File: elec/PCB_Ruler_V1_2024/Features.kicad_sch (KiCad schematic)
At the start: 4 parts

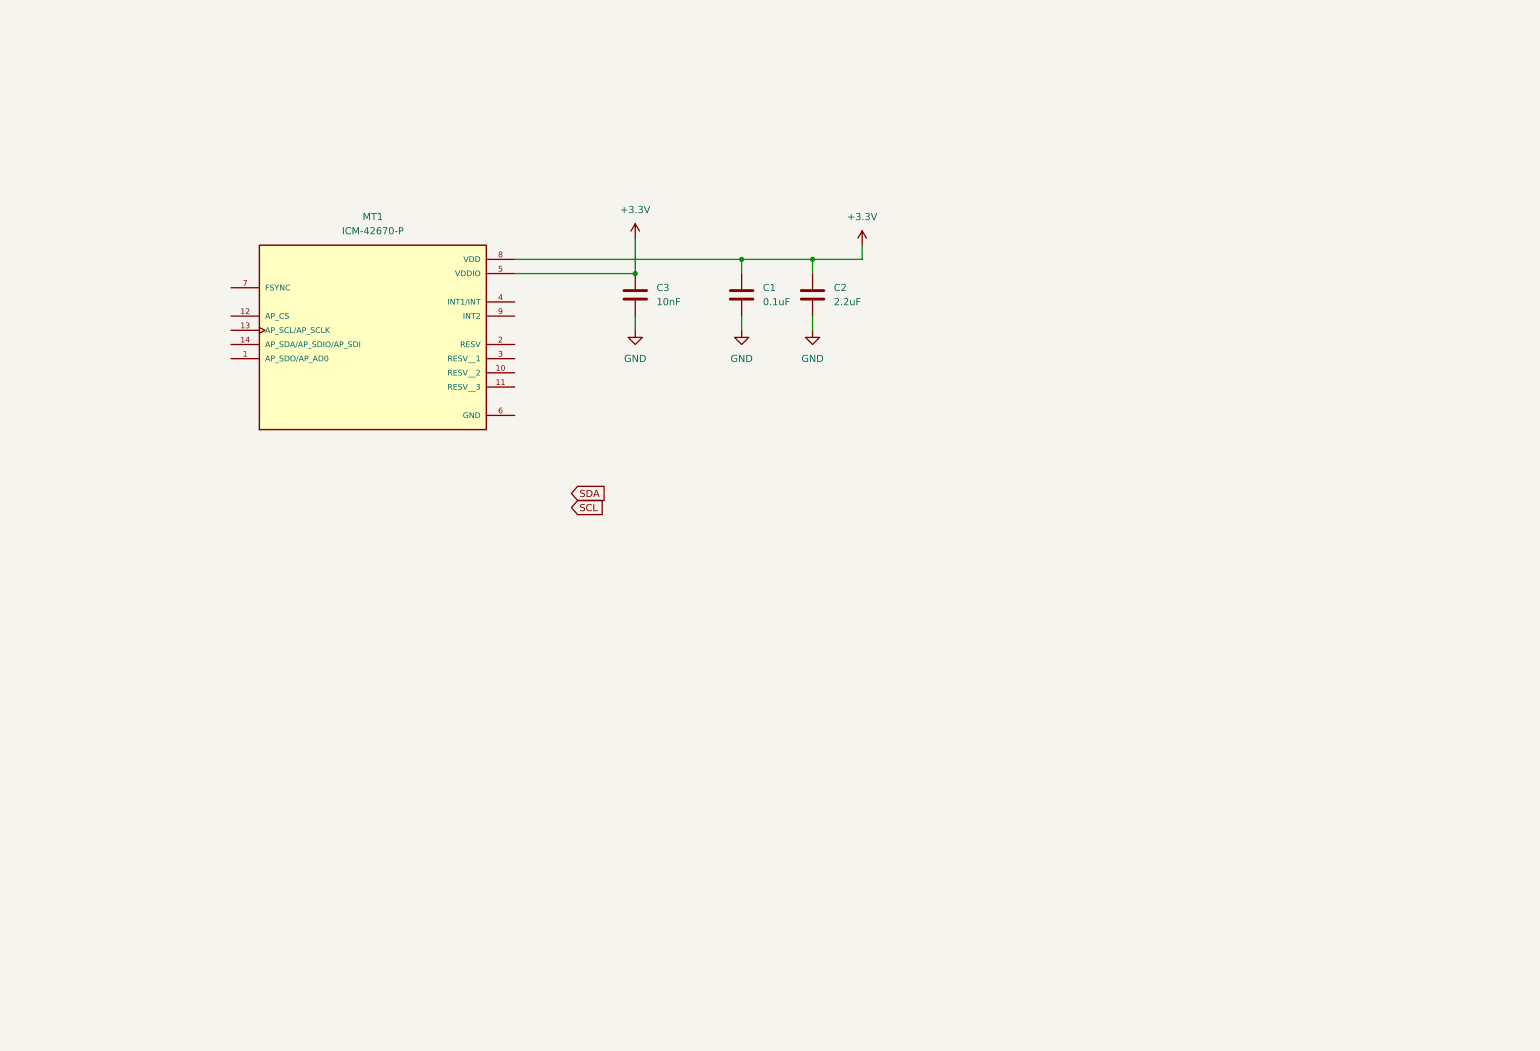
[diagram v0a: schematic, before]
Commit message: Laser
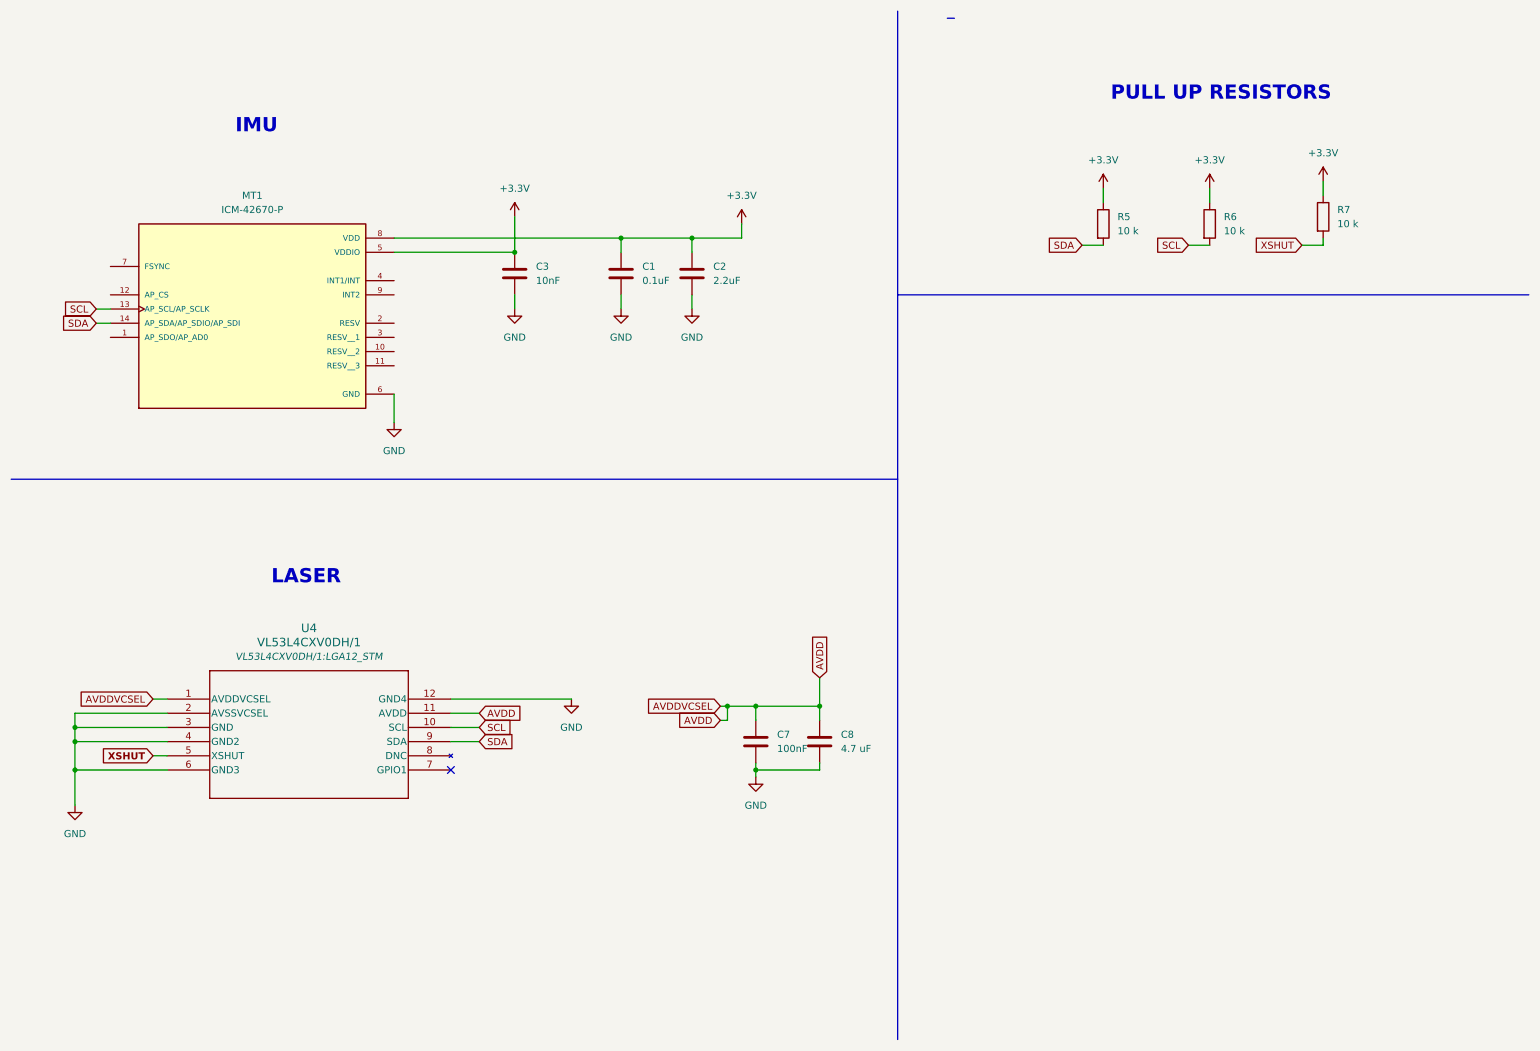
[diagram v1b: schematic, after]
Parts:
- added C7: 100nF, symbol Device:C
- added C8: 4.7 uF, symbol Device:C
- added R5, R6, R7: 10 k, symbol Device:R
- added U4: VL53L4CXV0DH/1, VL53L4CXV0DH/1:LGA12_STM, symbol VL53L4CXV0DH/1:VL53L4CXV0DH_1
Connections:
- net +3.3V: now also R5.1, R6.1, R7.1
- net GND: now also MT1.6 (GND), C7.2, C8.2, U4.12 (GND4), U4.2 (AVSSVCSEL), U4.3 (GND), U4.4 (GND2), U4.6 (GND3)
- net SCL: now also MT1.13 (AP_SCL/AP_SCLK), R6.2, U4.10 (SCL)
- net SDA: now also MT1.14 (AP_SDA/AP_SDIO/AP_SDI), R5.2, U4.9 (SDA)
- new net AVDD: C7.1, C8.1, U4.1 (AVDDVCSEL), U4.11 (AVDD)
- new net XSHUT: R7.2, U4.5 (XSHUT)
- no-connect marks 0 -> 1
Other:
- note added: "IMU"
- note added: "LASER"
- note added: "PULL UP RESISTORS"
- moved on the sheet: C1, C2, C3, MT1

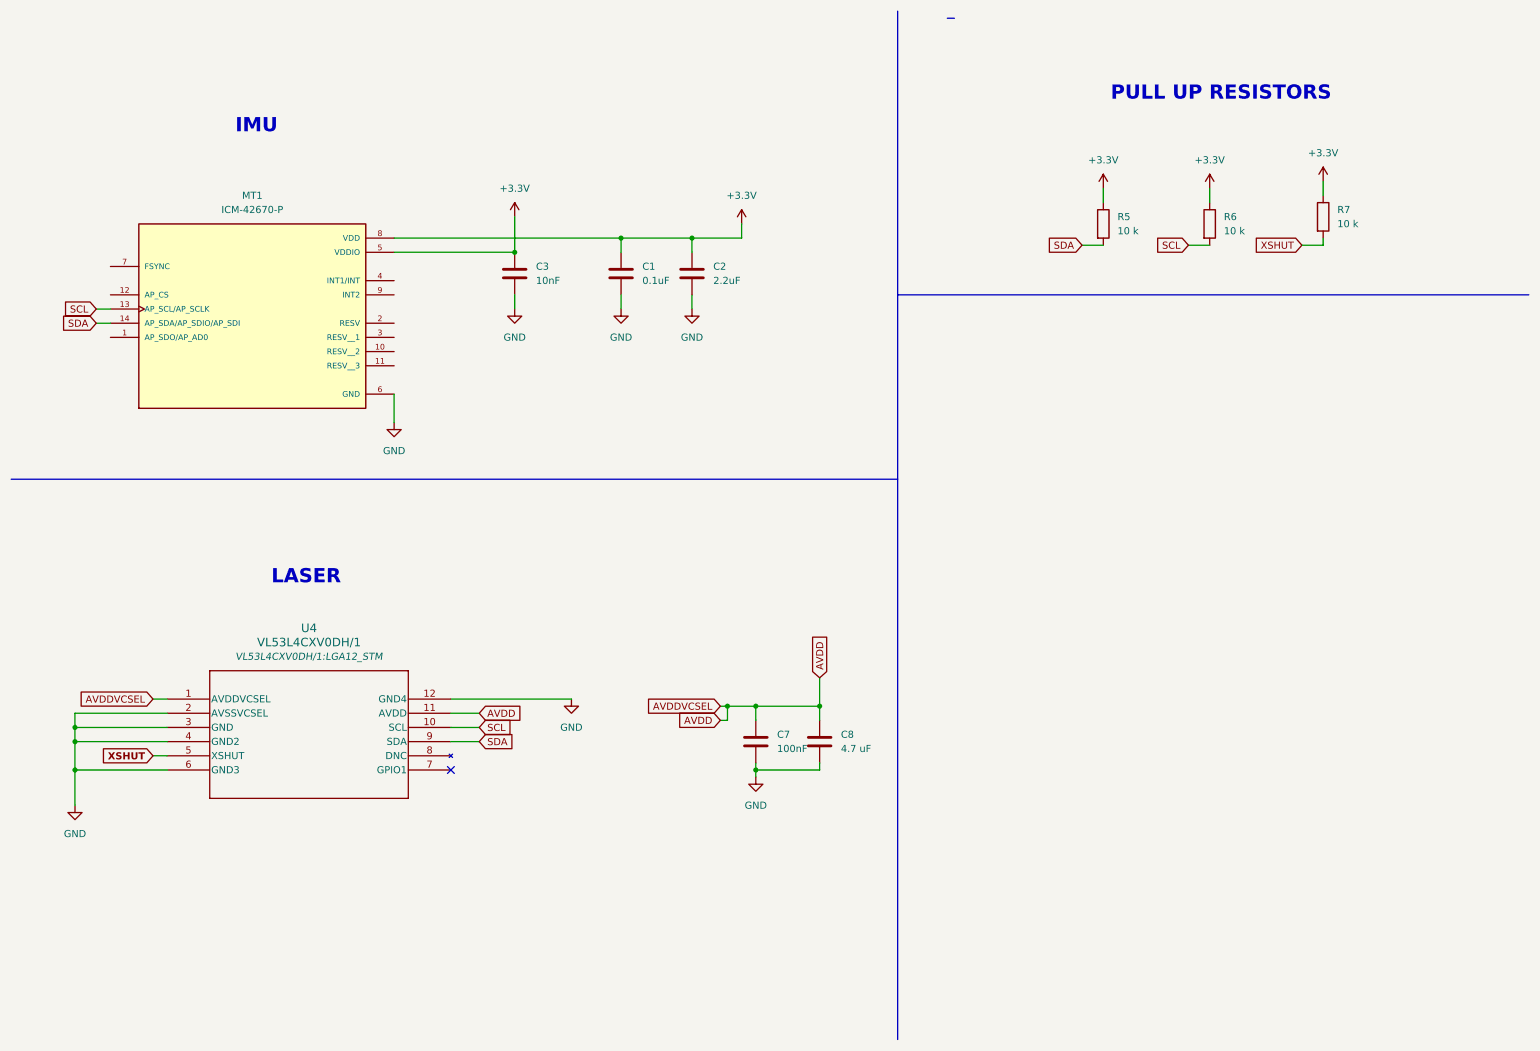
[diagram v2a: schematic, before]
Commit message: Almost finished schematic...
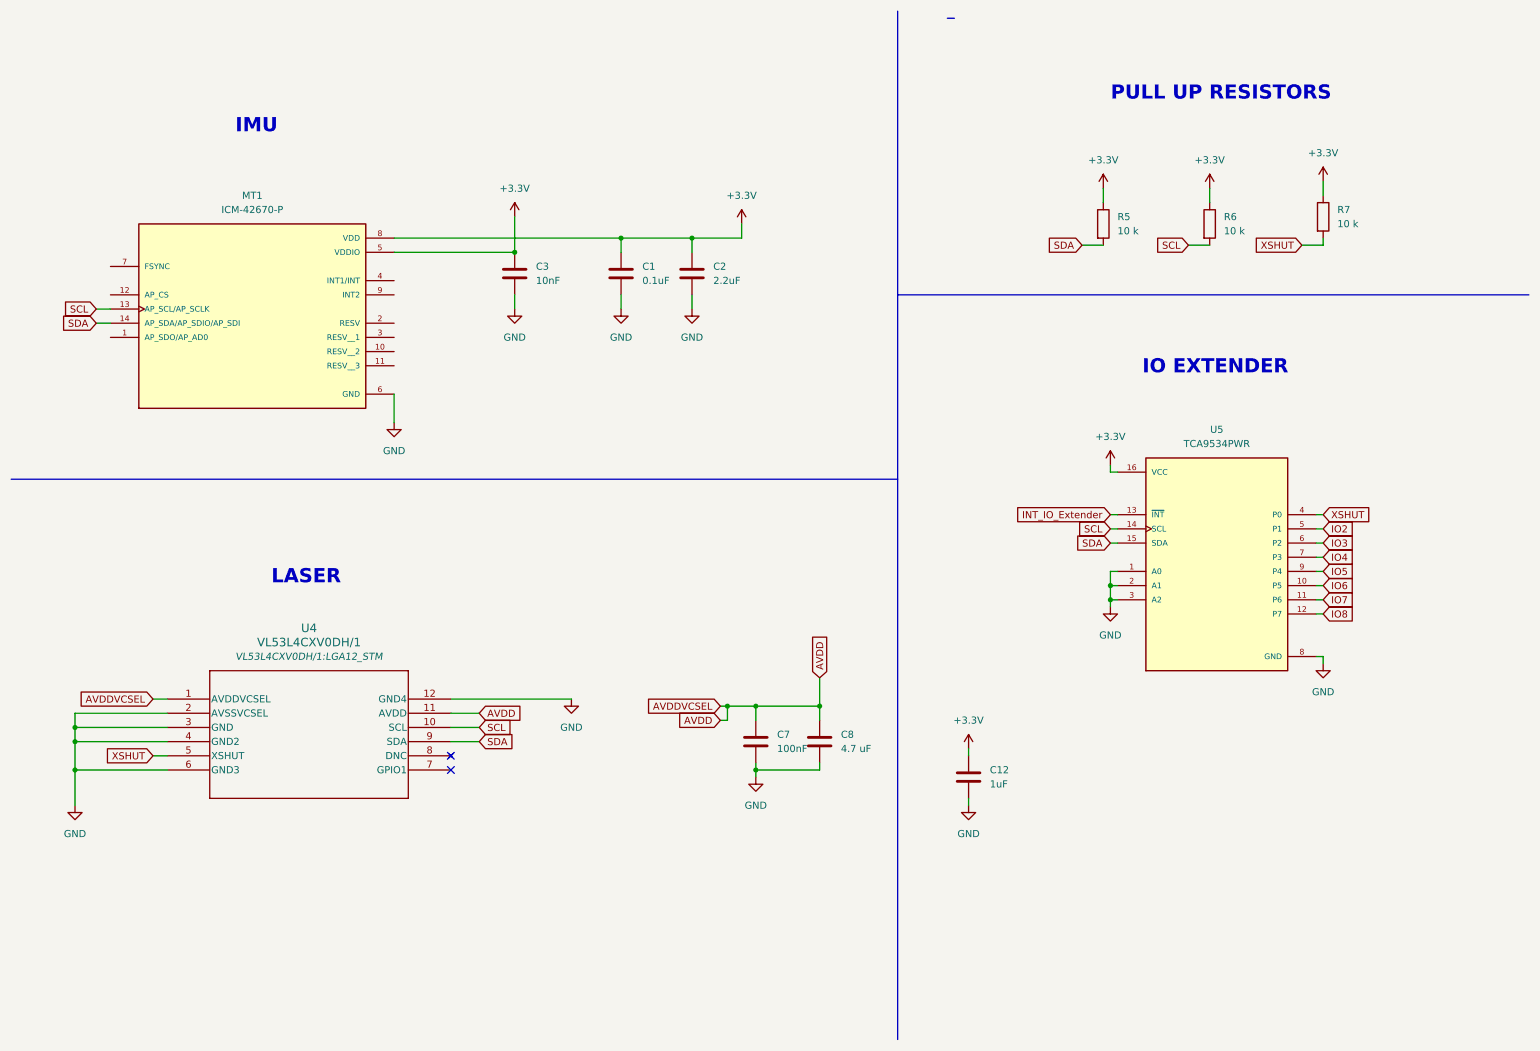
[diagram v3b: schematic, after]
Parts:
- added C12: 1uF, symbol Device:C
- added U5: TCA9534PWR, TCA9534PWR:SOP65P640X120-16N, symbol TCA9534PWR:TCA9534PWR
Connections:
- net +3.3V: now also C12.1, U5.16 (VCC)
- net GND: now also C12.2, U5.1 (A0), U5.2 (A1), U5.3 (A2), U5.8 (GND)
- net SCL: now also U5.14 (SCL)
- net SDA: now also U5.15 (SDA)
- net XSHUT: now also U5.4 (P0)
- new net INT_IO_Extender: U5.13 (~{INT})
- new net IO2: U5.5 (P1)
- new net IO3: U5.6 (P2)
- new net IO4: U5.7 (P3)
- new net IO5: U5.9 (P4)
- new net IO6: U5.10 (P5)
- new net IO7: U5.11 (P6)
- new net IO8: U5.12 (P7)
- no-connect marks 1 -> 2
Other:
- note added: "IO EXTENDER"

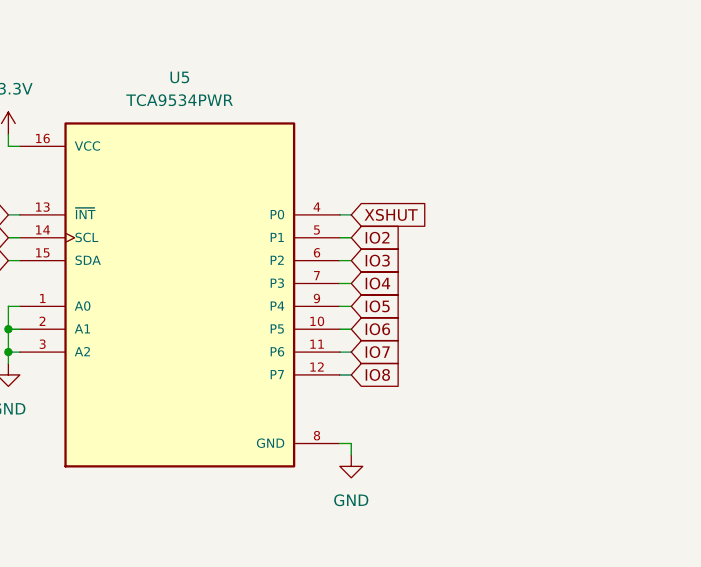
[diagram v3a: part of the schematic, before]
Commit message: protection and Buttons
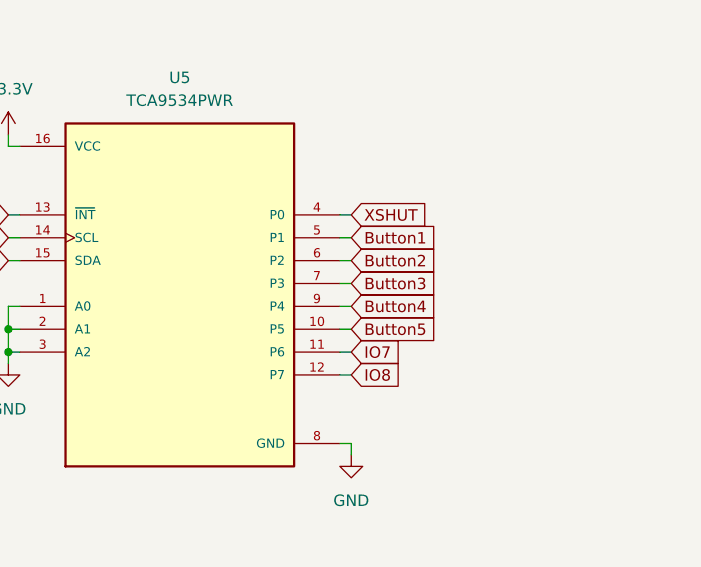
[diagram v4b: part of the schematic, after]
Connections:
- net IO2 renamed Button1
- net IO3 renamed Button2
- net IO4 renamed Button3
- net IO5 renamed Button4
- net IO6 renamed Button5
